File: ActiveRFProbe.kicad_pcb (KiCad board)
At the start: 2 copper layers, 50 x 21 mm, 41 parts, among them J1 Conn_01x01, J16 Conn_01x01, J17 Conn_01x01, J18 Conn_01x01, J19 Conn_01x01, J2 Conn_01x01, J20 Conn_01x01, J21 Conn_01x01, J22 Conn_01x01, J23 Conn_01x01, J24 Conn_01x01, J25 Conn_Coaxial, J3 Conn_01x01, Q1 2SC3357, Q2 2SC3357, Q3 2SC3357

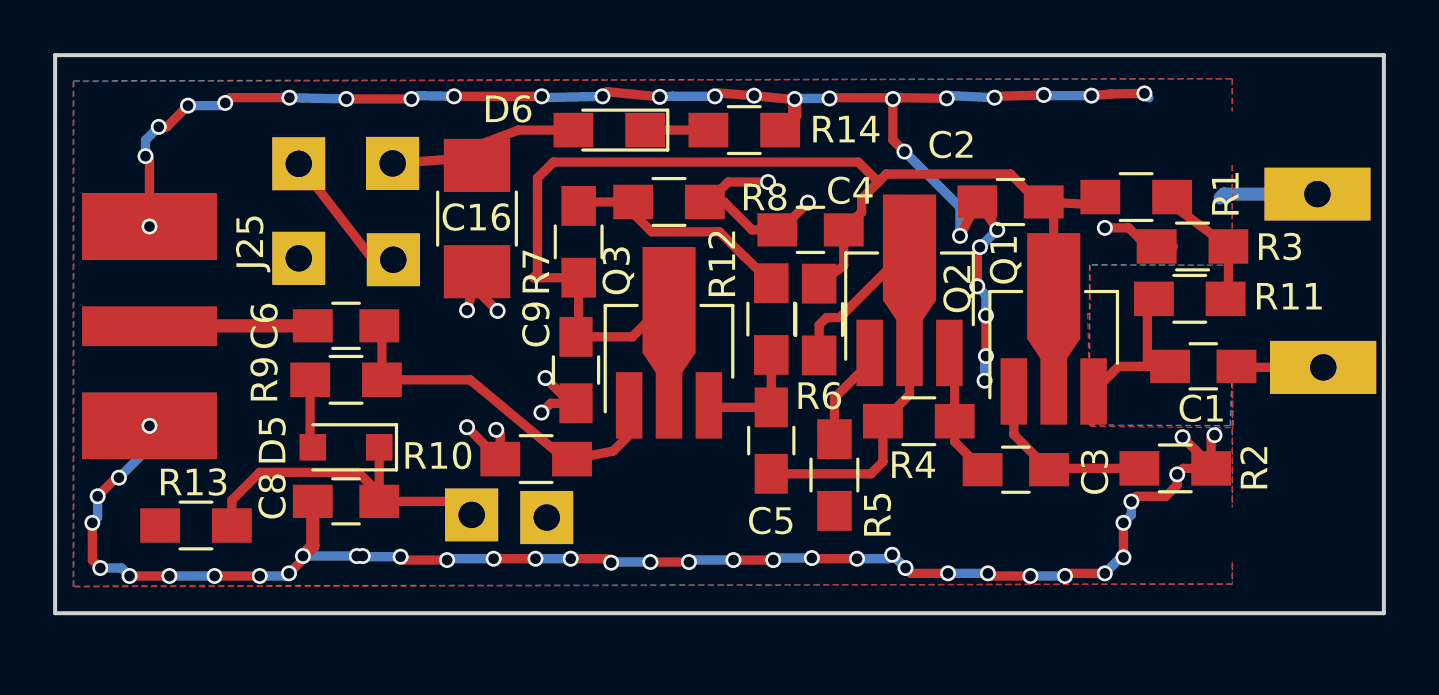
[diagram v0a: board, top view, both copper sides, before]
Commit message: Cleaned up the layout
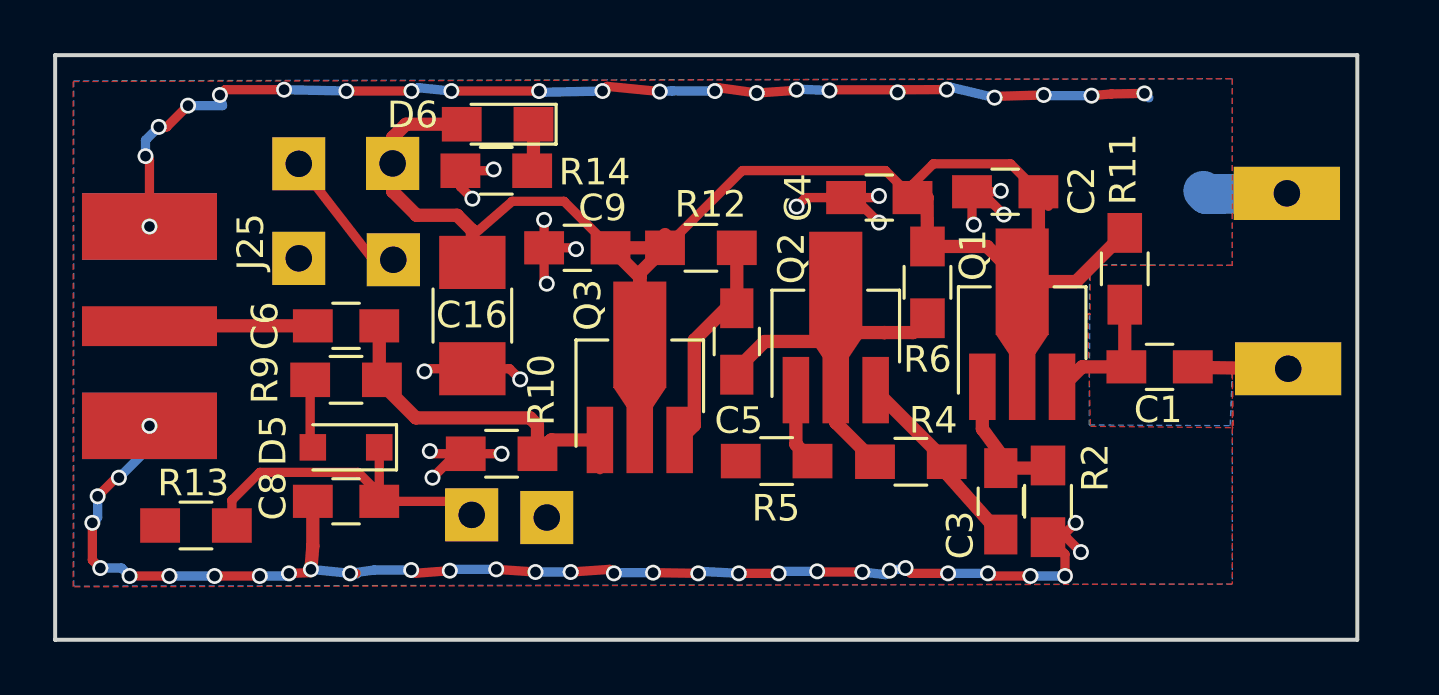
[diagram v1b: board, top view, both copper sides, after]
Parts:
- removed R1, R3: 10k, Resistors_SMD:R_0805_HandSoldering
- removed R7, R8: 1k, Resistors_SMD:R_0805_HandSoldering
- R11: value 10k -> 47k
- R12: value 1k -> 47k
- R5: value 0R -> 47R
- R6: value 220R -> 100R
- moved J23 14.3 mm to (87.9, 83.8)
- moved J21 14.1 mm to (88.0, 98.9)
- moved J20 13.1 mm to (95.2, 98.8)
- moved J22 12.7 mm to (95.5, 83.9)
- moved R14 9.46 mm to (81.6, 85.3), turned to 180 degrees
- moved R2 4.95 mm to (102.4, 97.8), turned to 270 degrees
- moved C9 4.60 mm to (84.7, 88.2), turned to 0 degrees
- moved R6 4.31 mm to (97.8, 89.5)
- moved D6 4.21 mm to (81.7, 83.6)
- moved C5 3.95 mm to (90.7, 91.8)
- moved R12 3.77 mm to (89.3, 88.2), turned to 180 degrees
- moved C16 3.65 mm to (80.7, 90.8)
- moved Q2 3.11 mm to (94.4, 91.6)
- moved C4 2.86 mm to (96.0, 86.4)
- moved R11 2.69 mm to (105.2, 89.0), turned to 90 degrees
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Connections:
- C16 pad 2: Net-(C16-Pad2) -> +9V
- D6 pad 2: Net-(C16-Pad2) -> +9V
- J2 pad 1: Net-(C16-Pad2) -> +9V
- R11 pad 2: Net-(R1-Pad2) -> +9V
- R12 pad 2: Net-(R12-Pad2) -> +9V
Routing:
- net +9V: track 52.8 -> 75.0 mm
- net GND: track 143.7 -> 124.5 mm, vias 77 -> 70
- net Net-(R12-Pad2): track 8.83 -> 0.00 mm
- net Net-(C16-Pad2): track 8.59 -> 0.00 mm
- net Net-(C5-Pad1): track 4.35 -> 9.39 mm
- net Net-(R1-Pad2): track 4.94 -> 0.00 mm
- net Net-(C5-Pad2): track 18.8 -> 15.7 mm
- net Net-(C3-Pad1): track 4.91 -> 7.60 mm
- net Net-(C3-Pad2): track 6.91 -> 5.11 mm
- net Net-(Q2-Pad1): track 5.16 -> 4.12 mm
- net Net-(D6-Pad1): track 2.38 -> 1.77 mm
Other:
- board size 50 x 21 mm -> 49 x 22 mm
- board text added: "ACTIVE RF PROBE BY D MARKS KW4TI CC-BY-SA 4.0"
- board text removed: "RF PROBE BY D MARKS KW4TI CC-BY-SA 4.0"
